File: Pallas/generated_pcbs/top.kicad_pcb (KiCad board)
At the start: 2 copper layers, 467.5 x 140 mm, 19 parts

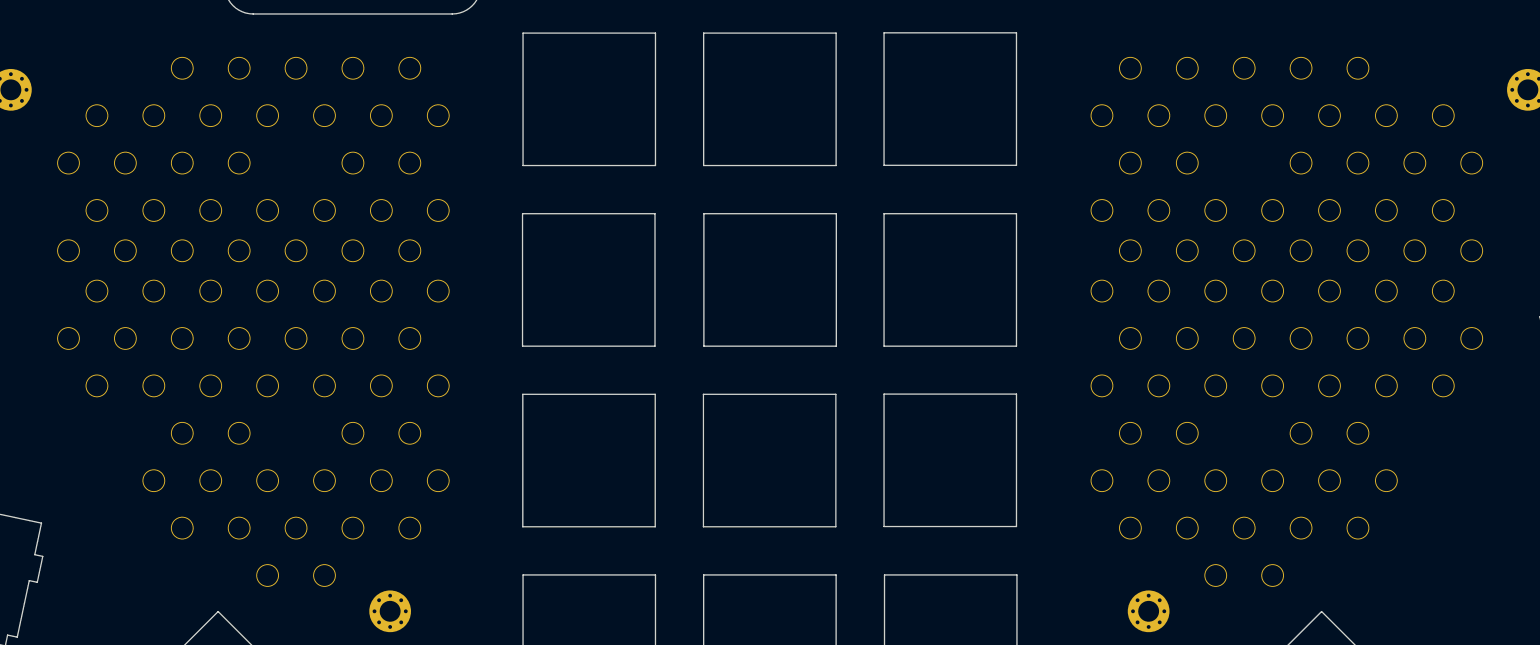
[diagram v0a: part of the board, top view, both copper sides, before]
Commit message: Pallas rev 0.3
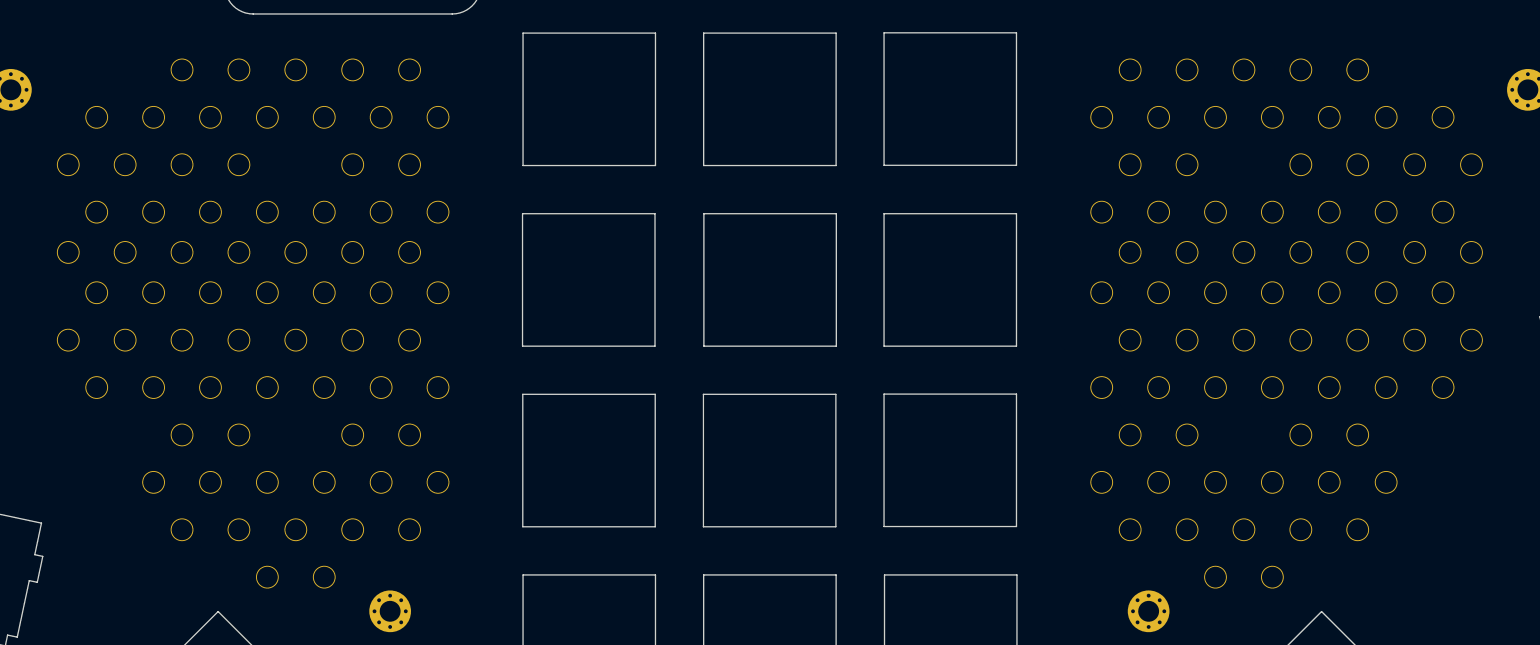
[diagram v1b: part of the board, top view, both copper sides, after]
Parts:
- moved DecorationHoleTop1 0.18 mm to (238.9, 114.3)
- moved DecorationHoleTop2 0.18 mm to (338.9, 114.3)
